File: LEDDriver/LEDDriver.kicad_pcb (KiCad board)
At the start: 2 copper layers, 39.4 x 41.9 mm, 16 parts, among them CON1 36V DC Power, P1 En, P2 ToLED, P3 To5V Power, Q1 Q_PMOS_GDS

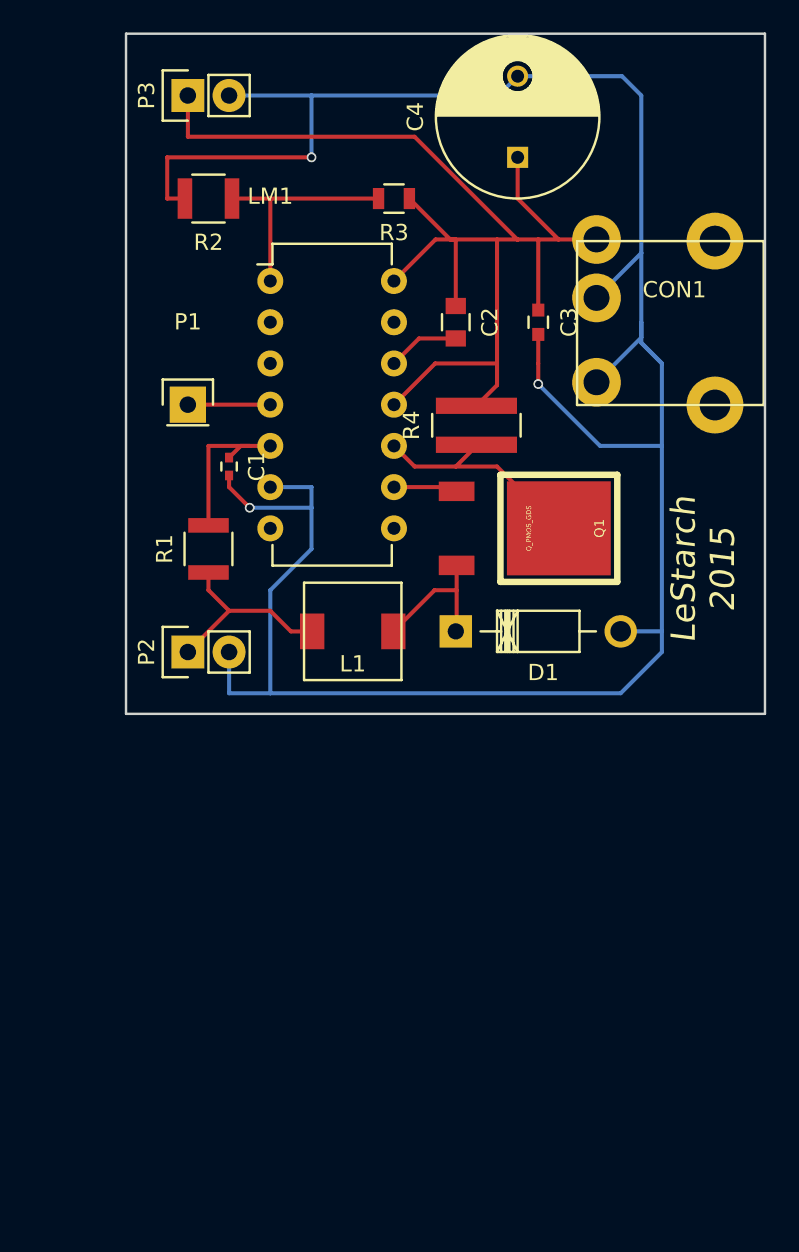
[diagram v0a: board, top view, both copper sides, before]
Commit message: lestarch: adding design files for combined design v2.0
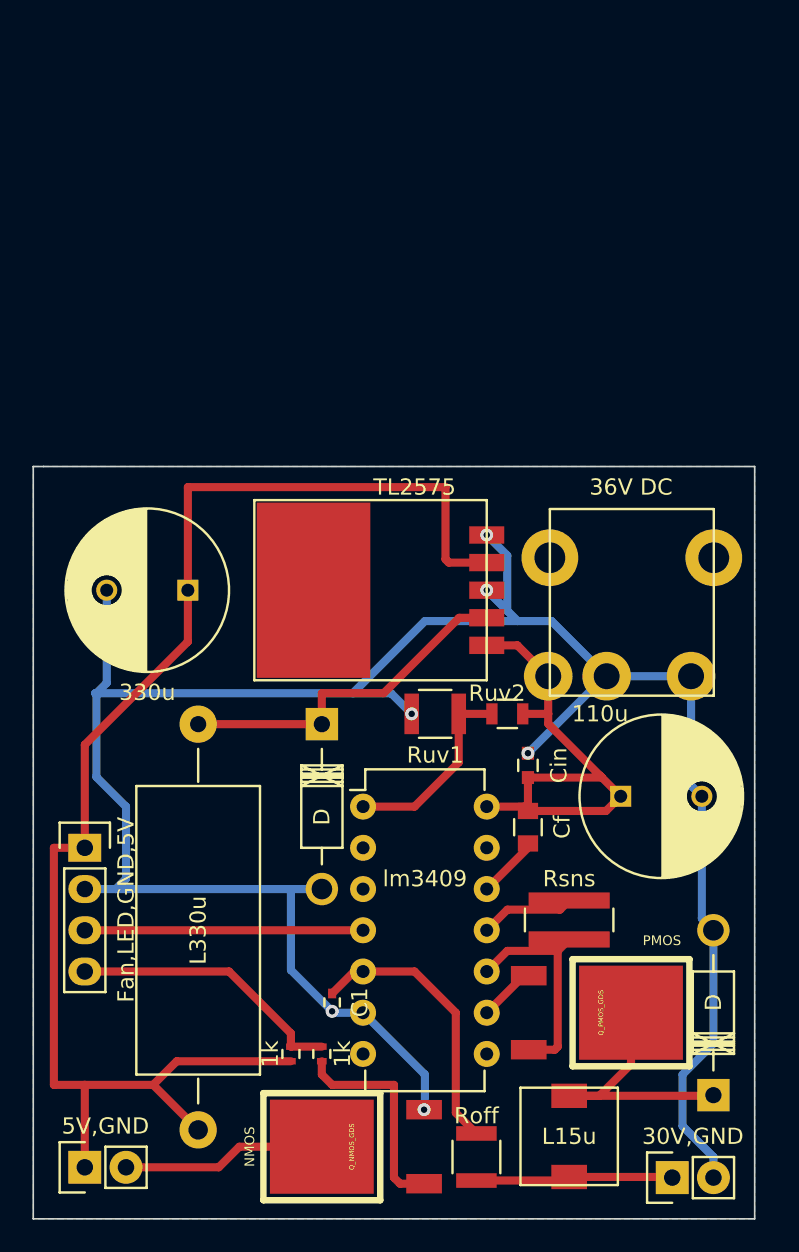
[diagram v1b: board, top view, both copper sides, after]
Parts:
- removed C2: Cf, Capacitors_SMD:C_0805
- removed C3: Cin, Capacitors_SMD:C_0603
- removed C4: CP, Capacitors_ThroughHole:C_Radial_D10_L16_P5
- removed CON1: 36V DC Power, footprints:PJ-051A
- removed D1: D_Schottky, Diodes_ThroughHole:Diode_DO-41_SOD81_Horizontal_RM10
- removed L1: INDUCTOR, footprints:SLF6045
- removed LM1: lm3409, Housings_DIP:DIP-14_W7.62mm
- removed P1: En, Pin_Headers:Pin_Header_Straight_1x01
- removed P2: ToLED, Pin_Headers:Pin_Header_Straight_1x02
- removed P3: To5V Power, Pin_Headers:Pin_Header_Straight_1x02
- removed Q1: Q_PMOS_GDS, footprints:TO-252-3
- removed R1: Roff, Resistors_SMD:R_1210
- removed R2: Ruv1, Resistors_SMD:R_1210
- removed R3: Ruv2, Resistors_SMD:R_0805
- removed R4: Rsns, footprints:R_1020
- added 110u: CP, Capacitors_ThroughHole:C_Radial_D10_L16_P5, F.Cu at (162.6, 88.9)
- added 1k: R, Resistors_SMD:R_0402, F.Cu at (142.2, 104.8)
- added 1k: R, Resistors_SMD:R_0402, F.Cu at (144.1, 104.8)
- added 30V,GND: ToLED, Pin_Headers:Pin_Header_Straight_1x02, F.Cu at (165.7, 112.4)
- added 330u: 330u, Capacitors_ThroughHole:C_Radial_D10_L16_P5, F.Cu at (135.9, 76.2)
- added 36V DC: 36V DC Power, footprints:PJ-051A, F.Cu at (163.2, 76.2)
- added 5V,GND: FanOut, Pin_Headers:Pin_Header_Straight_1x02, F.Cu at (129.5, 111.8)
- added Cf: Cf, Capacitors_SMD:C_0805, F.Cu at (156.8, 90.8)
- added Cin: Cin, Capacitors_SMD:C_0603, F.Cu at (156.8, 87.0)
- added D: D_Schottky, Diodes_ThroughHole:Diode_DO-41_SOD81_Horizontal_RM10, F.Cu at (168.3, 107.3)
- added D: D_Schottky, Diodes_ThroughHole:Diode_DO-41_SOD81_Horizontal_RM10, F.Cu at (144.1, 84.5)
- added Fan,LED,GND,5V: TeensyConnector, Pin_Headers:Pin_Header_Straight_1x04, F.Cu at (129.5, 92.1)
- added L15u: INDUCTOR, footprints:SLF6045, F.Cu at (159.4, 109.9)
- added L330u: 330u, Resistors_ThroughHole:Resistor_Horizontal_RM25mm, F.Cu at (136.5, 84.5)
- added NMOS: Q_NMOS_GDS, footprints:TO-252-3, F.Cu at (144.1, 110.5)
- added PMOS: Q_PMOS_GDS, footprints:TO-252-3, F.Cu at (163.2, 102.2)
- added Roff: Roff, Resistors_SMD:R_1210, F.Cu at (153.7, 111.1)
- added Rsns: Rsns, footprints:R_1020, F.Cu at (159.4, 96.5)
- added Ruv1: Ruv1, Resistors_SMD:R_1210, F.Cu at (151.1, 83.8)
- added Ruv2: Ruv2, Resistors_SMD:R_0805, F.Cu at (155.6, 83.8)
- added TL2575: TL25527, footprints:TO-263, F.Cu at (154.3, 76.2)
- added lm3409: lm3409, Housings_DIP:DIP-14_W7.62mm, F.Cu at (146.7, 89.5)
- moved C1 33.6 mm to (144.8, 101.6)
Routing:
- net /Regulator1/5VOut: track 0.00 -> 88.5 mm
- net VCC: track 75.7 -> 36.8 mm
- net Net-(D201-Pad1): track 0.00 -> 21.6 mm
- net Net-(P3-Pad4): track 0.00 -> 17.0 mm
- net Net-(Q2-Pad1): track 0.00 -> 13.3 mm
- net Net-(P1-Pad2): track 0.00 -> 12.6 mm
- net Net-(LM1-Pad4): track 5.08 -> 17.1 mm
- net GND: track 155.8 -> 147.2 mm, vias 3 -> 6
- net Net-(D1-Pad1): track 9.04 -> 16.7 mm
- net Net-(C1-Pad1): track 10.3 -> 17.2 mm
- net Net-(LM1-Pad1): track 14.1 -> 12.1 mm
- net Net-(C2-Pad2): track 4.45 -> 3.86 mm
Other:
- board size 39.4 x 41.9 mm -> 44.5 x 46.4 mm
- net class Default: trace_width 0.25 -> 0.5; via_dia 0.6 -> 0.8
- rule pad_to_mask_clearance: 0.2 -> 0
- board text added: "LeStarch 2016 - Combined circuit for micro- controller driven LED lamp. - LED Driver 30V, 1A - Regulator 5V, ~1A - NMOS GND switch"
- board text removed: "LED driver: Vin - 36V, Vout - 30V, Iout - 1A LEDs need a constant current and thus cannot be driven given just a voltage, but rather must be driven to maintain constant current."
- board text removed: "LeStarch 2015"
